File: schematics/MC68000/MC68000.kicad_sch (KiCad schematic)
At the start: 0 parts

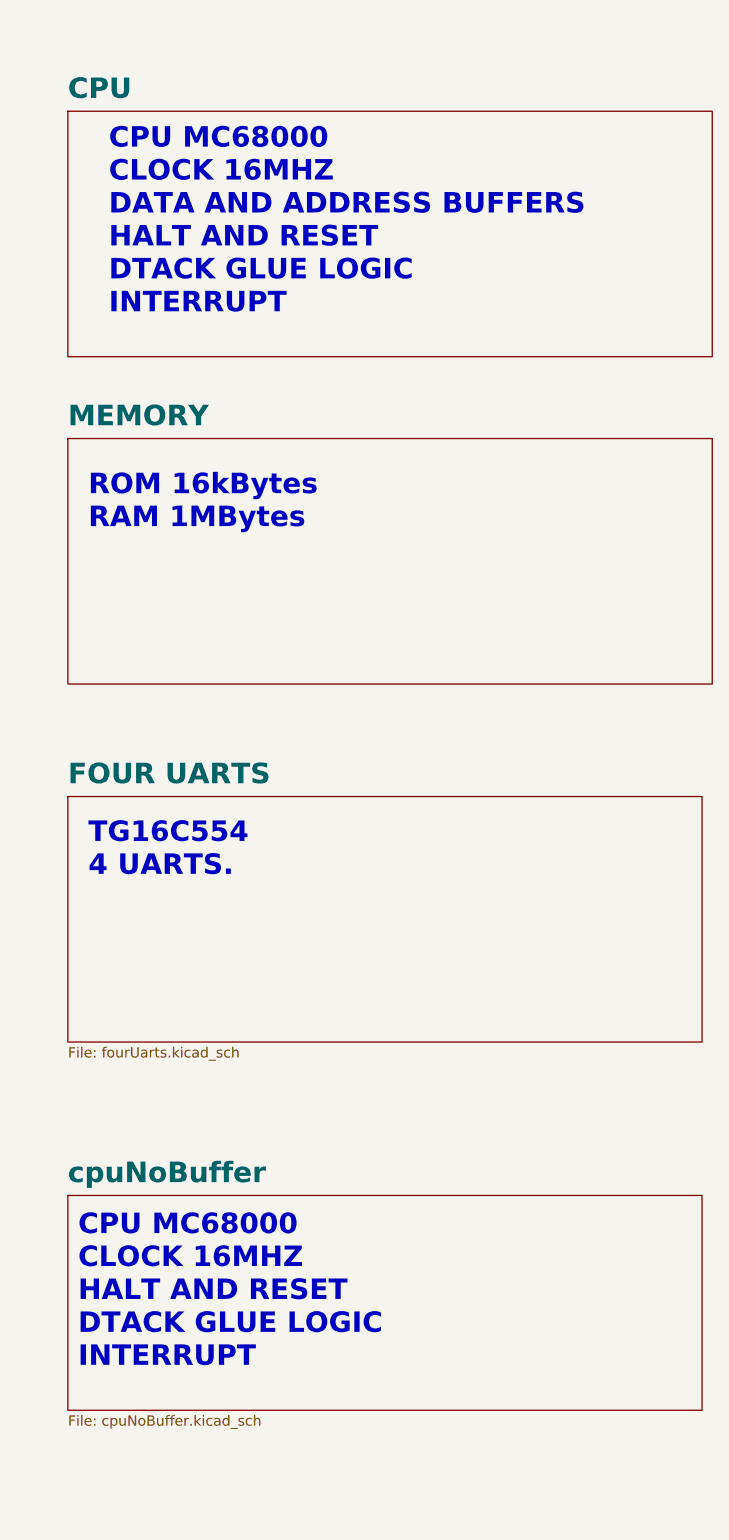
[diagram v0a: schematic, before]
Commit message: Ram memory test 2 OK
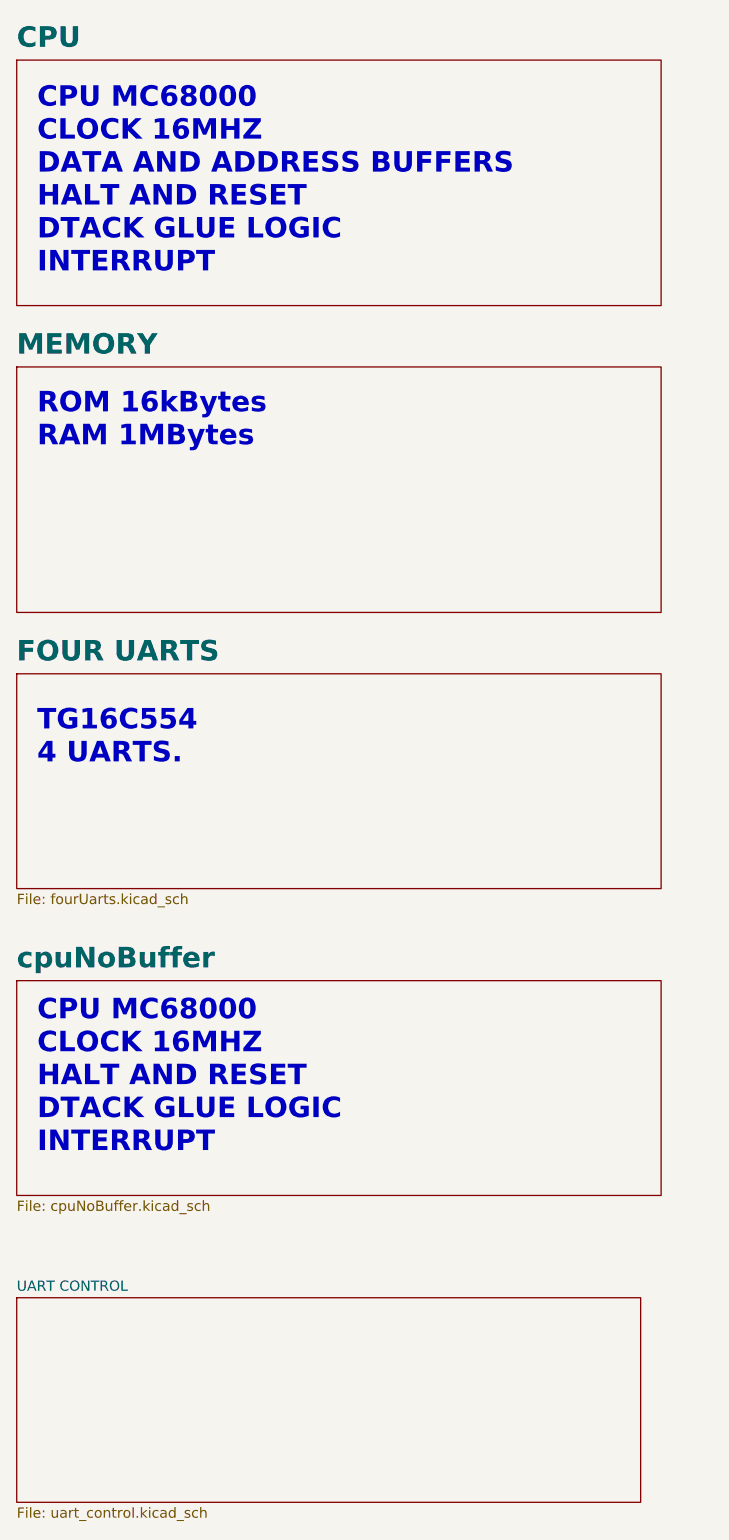
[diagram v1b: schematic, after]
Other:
- added sheet UART CONTROL (uart_control.kicad_sch)
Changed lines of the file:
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@@
 (kicad_sch (version 20230121) (generator eeschema)
   (paper "A3")
-  (text "ROM 16kBytes\nRAM 1MBytes\n" (at 34.29 83.82 0)
+  (text "ROM 16kBytes\nRAM 1MBytes\n" (at 27.94 73.66 0)
     (effects (font (size 2.54 2.54) (thickness 0.508) bold) (justify left bottom))
   )
   (text "CPU MC68000 \nCLOCK 16MHZ\nDATA AND ADDRESS BUFFERS\nHALT AND RESET\nDTACK GLUE LOGIC\nINTERRUPT "
-    (at 36.83 57.15 0)
+    (at 27.94 52.07 0)
     (effects (font (size 2.54 2.54) (thickness 0.254) bold) (justify left bottom))
   )
   (text "CPU MC68000 \nCLOCK 16MHZ\nHALT AND RESET\nDTACK GLUE LOGIC\nINTERRUPT "
-    (at 33.02 187.96 0)
+    (at 27.94 161.29 0)
     (effects (font (size 2.54 2.54) (thickness 0.508) bold) (justify left bottom))
   )
-  (text "TG16C554\n4 UARTS.\n" (at 34.29 127 0)
+  (text "TG16C554\n4 UARTS.\n" (at 27.94 113.03 0)
     (effects (font (size 2.54 2.54) (thickness 0.508) bold) (justify left bottom))
   )
-  (sheet (at 31.75 72.39) (size 80.01 30.48) (fields_autoplaced)
+  (sheet (at 25.4 63.5) (size 80.01 30.48) (fields_autoplaced)
     (stroke (width 0.1524) (type solid))
     (fill (color 0 0 0 0.0000))
-    (property "Sheetname" "MEMORY" (at 31.75 71.0434 0) (show_name)
+    (property "Sheetname" "MEMORY" (at 25.4 62.1534 0) (show_name)
       (effects (font (size 2.54 2.54) bold) (justify left bottom))
     )
-    (property "Sheetfile" "memory.kicad_sch" (at 31.75 103.4546 0)
+    (property "Sheetfile" "memory.kicad_sch" (at 25.4 94.5646 0)
       (effects (font (size 1.27 1.27)) (justify left top) hide)
     )
@@
     )
   )
-  (sheet (at 31.75 116.84) (size 78.74 30.48) (fields_autoplaced)
+  (sheet (at 25.4 101.6) (size 80.01 26.67) (fields_autoplaced)
     (stroke (width 0.1524) (type solid))
     (fill (color 0 0 0 0.0000))
-    (property "Sheetname" "FOUR UARTS" (at 31.75 115.4934 0) (show_name)
+    (property "Sheetname" "FOUR UARTS" (at 25.4 100.2534 0) (show_name)
       (effects (font (size 2.54 2.54) bold) (justify left bottom))
     )
-    (property "Sheetfile" "fourUarts.kicad_sch" (at 31.75 147.9046 0)
+    (property "Sheetfile" "fourUarts.kicad_sch" (at 25.4 128.8546 0)
       (effects (font (size 1.27 1.27)) (justify left top))
     )
@@
     )
   )
-  (sheet (at 31.75 31.75) (size 80.01 30.48) (fields_autoplaced)
+  (sheet (at 25.4 25.4) (size 80.01 30.48) (fields_autoplaced)
     (stroke (width 0.1524) (type solid))
     (fill (color 0 0 0 0.0000))
-    (property "Sheetname" "CPU" (at 31.75 30.4034 0) (show_name)
+    (property "Sheetname" "CPU" (at 25.4 24.0534 0) (show_name)
       (effects (font (size 2.54 2.54) bold) (justify left bottom))
     )
-    (property "Sheetfile" "cpu.kicad_sch" (at 31.75 62.8146 0)
+    (property "Sheetfile" "cpu.kicad_sch" (at 25.4 56.4646 0)
       (effects (font (size 1.27 1.27)) (justify left top) hide)
     )
@@
     )
   )
-  (sheet (at 31.75 166.37) (size 78.74 26.67) (fields_autoplaced)
+  (sheet (at 25.4 179.07) (size 77.47 25.4) (fields_autoplaced)
     (stroke (width 0.1524) (type solid))
     (fill (color 0 0 0 0.0000))
-    (property "Sheetname" "cpuNoBuffer" (at 31.75 165.0234 0) (show_name)
+    (property "Sheetname" "UART CONTROL" (at 25.4 178.3584 0)
+      (effects (font (size 1.27 1.27)) (justify left bottom))
+    )
+    (property "Sheetfile" "uart_control.kicad_sch" (at 25.4 205.0546 0)
+      (effects (font (size 1.27 1.27)) (justify left top))
+    )
+    (instances
+      (project "MC68000"
+        (path "/99c9748a-87b3-41bd-bdc2-3a5f137c7a40" (page "6"))
+      )
+    )
+  )
+  (sheet (at 25.4 139.7) (size 80.01 26.67) (fields_autoplaced)
+    (stroke (width 0.1524) (type solid))
+    (fill (color 0 0 0 0.0000))
+    (property "Sheetname" "cpuNoBuffer" (at 25.4 138.3534 0) (show_name)
       (effects (font (size 2.54 2.54) bold) (justify left bottom))
     )
-    (property "Sheetfile" "cpuNoBuffer.kicad_sch" (at 31.75 193.6246 0)
+    (property "Sheetfile" "cpuNoBuffer.kicad_sch" (at 25.4 166.9546 0)
       (effects (font (size 1.27 1.27)) (justify left top))
     )
